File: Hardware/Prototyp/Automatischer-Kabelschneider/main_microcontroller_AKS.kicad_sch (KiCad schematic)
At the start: 34 parts, among them J3 Conn_01x04, J4 Conn_02x05_Odd_Even, J5 Conn_01x04, Q3 Q_NMOS_GSD, Q4 Q_NMOS_GSD, SW1 SW_Push, SW2 SW_Push, U5 TMC2209_SILENTSTEPSTICK, U6 ESP32-S3-WROOM-2, U7 TMC2209_SILENTSTEPSTICK

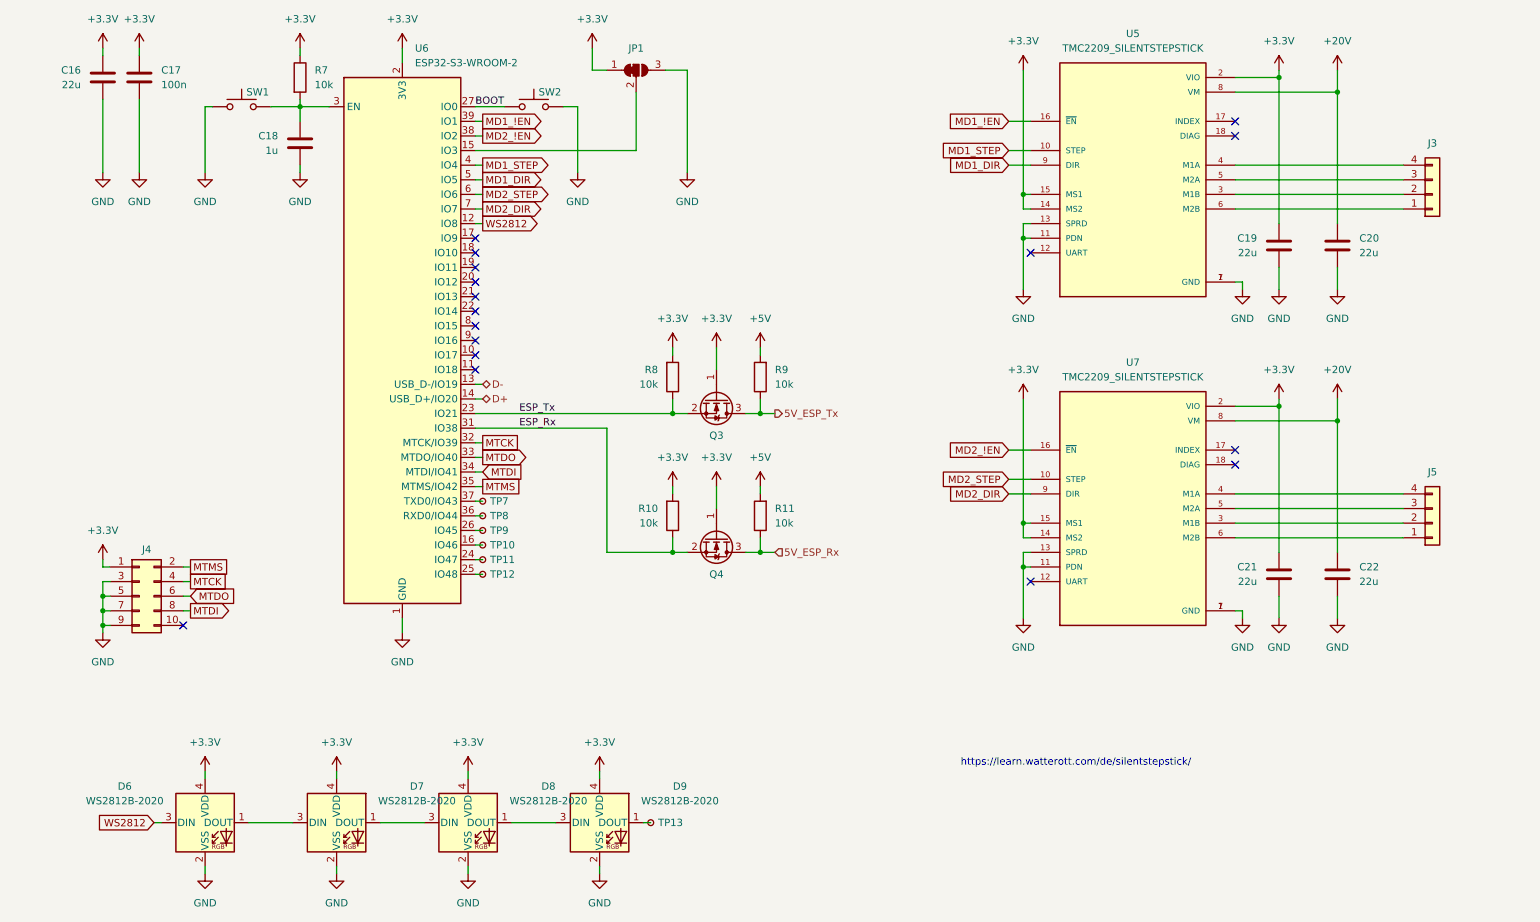
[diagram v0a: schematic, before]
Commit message: PCB finished
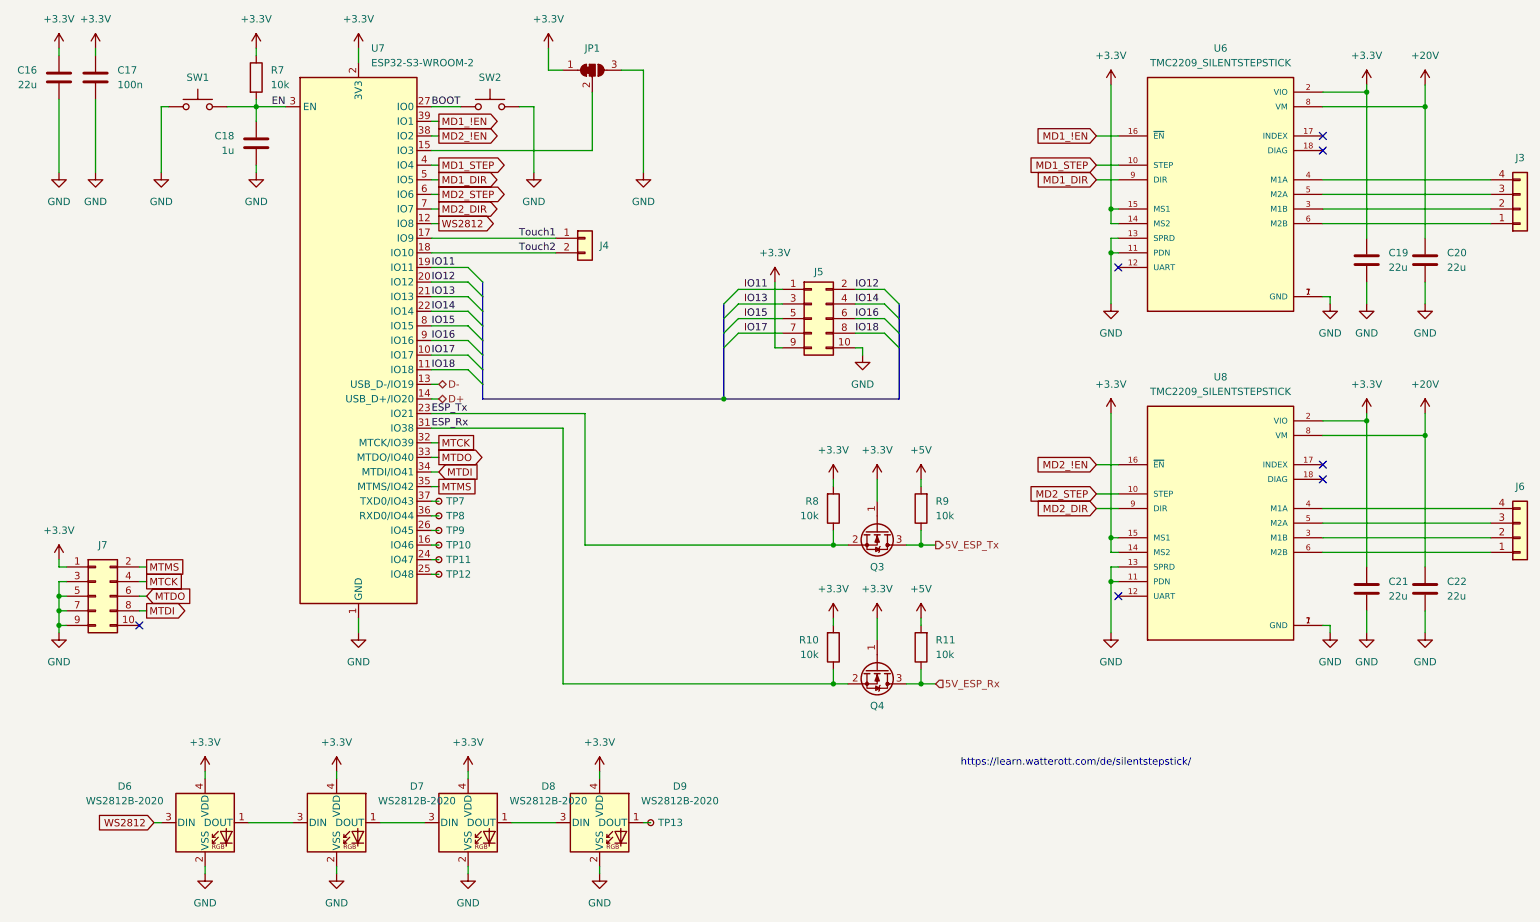
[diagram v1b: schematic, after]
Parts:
- added J4: Conn_01x02, Connector_Wire:SolderWire-1.5sqmm_1x02_P6mm_D1.7mm_OD3mm_Relief, symbol Connector_Generic:Conn_01x02
- added J5: Conn_02x05_Odd_Even, Connector_IDC:IDC-Header_2x05_P2.54mm_Vertical, symbol Connector_Generic:Conn_02x05_Odd_Even
- renumbered J5 to J6, J4 to J7, U5 to U6, U6 to U7, U7 to U8
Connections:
- net +3.3V: now also J5.9 (Pin_9)
- net GND: now also J5.10 (Pin_10)
- net IO17: now reaches U7.10 (IO17)
- net IO17: now also J5.7 (Pin_7)
- net IO18: now reaches U7.11 (IO18)
- net IO18: now also J5.8 (Pin_8)
- net Touch1: now reaches U7.17 (IO9)
- net Touch1: now also J4.1 (Pin_1)
- net Touch2: now reaches U7.18 (IO10)
- net Touch2: now also J4.2 (Pin_2)
- net IO11: now reaches U7.19 (IO11)
- net IO11: now also J5.1 (Pin_1)
- net IO12: now reaches U7.20 (IO12)
- net IO12: now also J5.2 (Pin_2)
- net IO13: now reaches U7.21 (IO13)
- net IO13: now also J5.3 (Pin_3)
- net IO14: now reaches U7.22 (IO14)
- net IO14: now also J5.4 (Pin_4)
- net EN: now reaches C18.1, R7.2, SW1.2, U7.3 (EN)
- net IO15: now reaches U7.8 (IO15)
- net IO15: now also J5.5 (Pin_5)
- net IO16: now reaches U7.9 (IO16)
- net IO16: now also J5.6 (Pin_6)
- no-connect marks 17 -> 7
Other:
- moved on the sheet: C16, C17, C18, C19, C20, C21, C22, J3, J6, J7, JP1, Q3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
